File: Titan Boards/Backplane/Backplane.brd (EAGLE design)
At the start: 195.1 x 76.2 mm, 29 parts, among them P1 39-30-02?_S, P3 39-30-04?_S

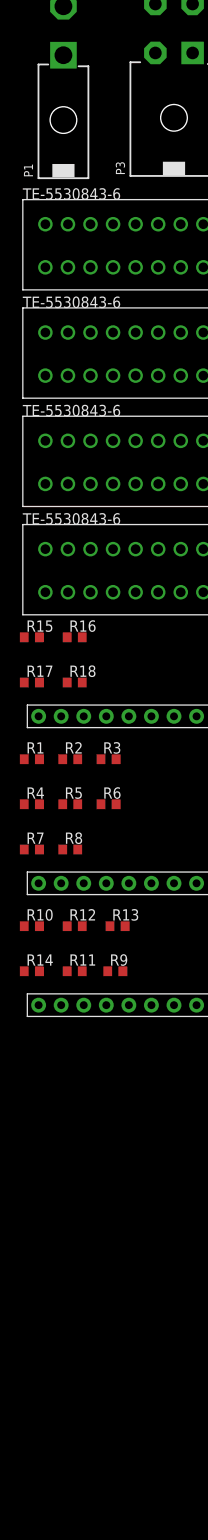
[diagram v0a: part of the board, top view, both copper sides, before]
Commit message: First final version of Titan Backplane Schematic
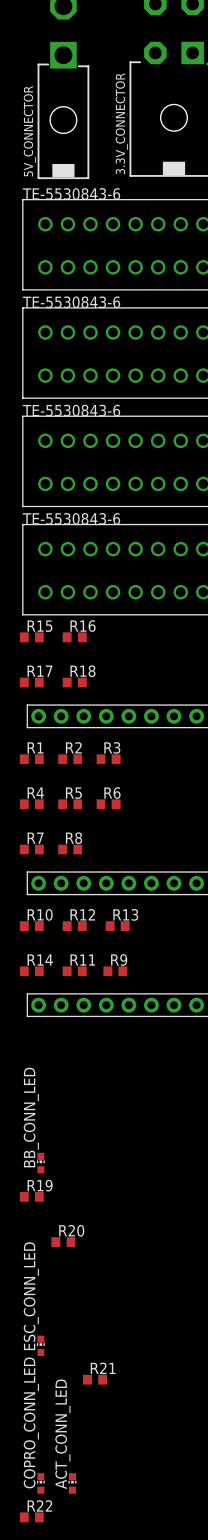
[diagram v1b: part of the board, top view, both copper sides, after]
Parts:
- added ACT_CONN_LED, BB_CONN_LED, COPRO_CONN_LED, ESC_CONN_LED: (no value), led:CHIP-LED0603
- added R19, R20, R21, R22: 36, rcl:R0603
- renumbered P1 to 5V_CONNECTOR, P3 to 3.3V_CONNECTOR, U$5 to KILLSWITCH_CONNECTOR, U$6 to THRUSTER_CONNECTOR, U$7 to ENABLE_SIGNALS_CONNECTOR, U$8 to I2C_CONNECTOR
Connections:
- removed net SPARE7: KILLSWITCH_CONNECTOR.P$1, U$1.43, U$2.43, U$3.43, U$4.43
- new net ACT_CONN: ACT_CONN_LED.A, U$4.43
- new net BB_CONN: BB_CONN_LED.A, U$1.43
- new net COPRO_CONN: COPRO_CONN_LED.A, U$3.43
- new net ESC_CONN: ESC_CONN_LED.A, U$2.43
- new net N$12: BB_CONN_LED.C, R19.1
- new net N$13: ESC_CONN_LED.C, R20.1
- new net N$14: COPRO_CONN_LED.C, R21.1
- new net N$15: ACT_CONN_LED.C, R22.1
- net GND: now also R19.2, R20.2, R21.2, R22.2

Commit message: Titan Backplane Final Version 1
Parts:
- removed 3.3V_CONNECTOR: 39-30-04?_S, con-molex-mini-fit:39-30-?04?
- removed ENABLE_SIGNALS_CONNECTOR: 929870-01-09_3, 3M_929852_Connector:929852-01-09_1ROW
- removed I2C_CONNECTOR: 929870-01-09_4, 3M_929852_Connector:929852-01-09_1ROW
- removed KILLSWITCH_CONNECTOR: 929870-01-09_1, 3M_929852_Connector:929852-01-09_1ROW
- removed R1, R10, R11, R12, R13, R14, R2, R3, R4, R5, R6, R7, R8, R9: 10k, rcl:R0603
- removed THRUSTER_CONNECTOR: 929870-01-09_2, 3M_929852_Connector:929852-01-09_1ROW
- added AUX_I2C_CONNECTOR1, ROBOT_I2C_CONNECTOR: 39-30-04?_S, con-molex-mini-fit:39-30-?04?
- added TESTPIN_CONNECTOR: 929870-01-09_4, 3M_929852_Connector:929852-01-09_1ROW
- SWITCH_CONNECTOR: value 39-30-08?_S -> 39-30-02?_S; device con-molex-mini-fit:39-30-?08? -> con-molex-mini-fit:39-30-?02?
- moved COPRO_CONN_LED 763.8 mm to (88.5, 58.7)
- moved R21 751.4 mm to (90.4, 58.3), turned to 270 degrees
- moved R19 736.0 mm to (119.1, 58.5), turned to 270 degrees
- moved BB_CONN_LED 732.3 mm to (121.0, 58.4)
- moved R22 727.9 mm to (90.3, 18.4), turned to 270 degrees
- moved ACT_CONN_LED 723.2 mm to (88.5, 18.2)
- moved ESC_CONN_LED 712.5 mm to (121.0, 17.8)
- moved R20 700.3 mm to (119.3, 17.8), turned to 270 degrees
- moved U$3 643.8 mm to (16.5, 55.9)
- moved U$1 631.0 mm to (124.5, 55.9)
- moved R17 616.9 mm to (54.7, 4.45), turned to 270 degrees
- moved R18 616.7 mm to (57.3, 4.45), turned to 270 degrees
- moved U$4 615.3 mm to (16.5, 15.2)
- moved R15 611.4 mm to (49.7, 4.45), turned to 270 degrees
- moved R16 611.2 mm to (52.2, 4.45), turned to 270 degrees
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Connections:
- net 12V_ON/OFF: no longer ENABLE_SIGNALS_CONNECTOR.P$3
- net 3.3V: now also AUX_I2C_CONNECTOR1.1, ROBOT_I2C_CONNECTOR.1, TESTPIN_CONNECTOR.P$7; no longer 3.3V_CONNECTOR.1, I2C_CONNECTOR.P$7, R10.1, R11.1, R12.1, R13.1, R14.1, R9.1
- net 3.3V_ON/OFF: no longer ENABLE_SIGNALS_CONNECTOR.P$1
- net 5V: now also SWITCH_CONNECTOR.1, TESTPIN_CONNECTOR.P$9; no longer I2C_CONNECTOR.P$9, R1.1, R2.1, R3.1, R4.1, R5.1, R6.1, R7.1, R8.1
- net 5V_ON/OFF: no longer ENABLE_SIGNALS_CONNECTOR.P$2
- net ACOUSTIC_ON/OFF: no longer ENABLE_SIGNALS_CONNECTOR.P$4
- net BACKPLANE_SCL: now also TESTPIN_CONNECTOR.P$4; no longer I2C_CONNECTOR.P$4
- net BACKPLANE_SDA: now also TESTPIN_CONNECTOR.P$3; no longer I2C_CONNECTOR.P$3
- net CONTROL_SIGNAL: no longer ENABLE_SIGNALS_CONNECTOR.P$7
- net GND: now also AUX_I2C_CONNECTOR1.3, ROBOT_I2C_CONNECTOR.3, SWITCH_CONNECTOR.2, TESTPIN_CONNECTOR.P$8; no longer 3.3V_CONNECTOR.3, ENABLE_SIGNALS_CONNECTOR.P$9, I2C_CONNECTOR.P$8, SWITCH_CONNECTOR.5
- net JETSON_ON/OFF: no longer ENABLE_SIGNALS_CONNECTOR.P$5
- net KILL_SWITCH: no longer KILLSWITCH_CONNECTOR.P$7, R9.2, SWITCH_CONNECTOR.2
- net MOBO_ON/OFF: no longer ENABLE_SIGNALS_CONNECTOR.P$6
- net PLTA_ON/OFF: no longer ENABLE_SIGNALS_CONNECTOR.P$8, SWITCH_CONNECTOR.1
- net PWM_1: no longer R1.2, THRUSTER_CONNECTOR.P$9
- net PWM_2: no longer R2.2, THRUSTER_CONNECTOR.P$8
- net PWM_3: no longer R3.2, THRUSTER_CONNECTOR.P$7
- net PWM_4: no longer R4.2, THRUSTER_CONNECTOR.P$6
- net PWM_5: no longer R5.2, THRUSTER_CONNECTOR.P$5
- net PWM_6: no longer R6.2, THRUSTER_CONNECTOR.P$4
- net PWM_7: no longer R7.2, THRUSTER_CONNECTOR.P$3
- net PWM_8: no longer R8.2, THRUSTER_CONNECTOR.P$2
- net ROBOT_SCL: now also AUX_I2C_CONNECTOR1.4, ROBOT_I2C_CONNECTOR.4, TESTPIN_CONNECTOR.P$6; no longer 3.3V_CONNECTOR.4, I2C_CONNECTOR.P$6
- net ROBOT_SDA: now also AUX_I2C_CONNECTOR1.2, ROBOT_I2C_CONNECTOR.2, TESTPIN_CONNECTOR.P$5; no longer 3.3V_CONNECTOR.2, I2C_CONNECTOR.P$5
- net SPARE2: no longer THRUSTER_CONNECTOR.P$1
- net SPARE3: now also TESTPIN_CONNECTOR.P$2; no longer I2C_CONNECTOR.P$2
- net SPARE4: now also TESTPIN_CONNECTOR.P$1; no longer I2C_CONNECTOR.P$1
- net SPARE5: no longer KILLSWITCH_CONNECTOR.P$9
- net SPARE6: no longer KILLSWITCH_CONNECTOR.P$8
- net SWITCH_1: no longer KILLSWITCH_CONNECTOR.P$6, R10.2, SWITCH_CONNECTOR.3
- net SWITCH_2: no longer KILLSWITCH_CONNECTOR.P$5, R11.2, SWITCH_CONNECTOR.4
- net SWITCH_3: no longer KILLSWITCH_CONNECTOR.P$4, R12.2, SWITCH_CONNECTOR.6
- net SWITCH_4: no longer KILLSWITCH_CONNECTOR.P$3, R13.2, SWITCH_CONNECTOR.7
- net SWITCH_5: no longer KILLSWITCH_CONNECTOR.P$2, R14.2, SWITCH_CONNECTOR.8
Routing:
- net GND: track 0.00 -> 479.0 mm, vias 0 -> 8
- net 3.3V: track 0.00 -> 335.0 mm, vias 0 -> 2
- net ROBOT_SDA: track 0.00 -> 316.8 mm, vias 0 -> 5
- net 5V: track 0.00 -> 316.1 mm, vias 0 -> 3
- net ROBOT_SCL: track 0.00 -> 311.8 mm, vias 0 -> 2
- net BACKPLANE_SDA: track 0.00 -> 296.1 mm, vias 0 -> 5
- net BACKPLANE_SCL: track 0.00 -> 295.3 mm, vias 0 -> 5
- net SPARE4: track 0.00 -> 279.8 mm, vias 0 -> 4
- net SPARE3: track 0.00 -> 279.0 mm, vias 0 -> 4
- net PLTA_ON/OFF: track 0.00 -> 273.3 mm, vias 0 -> 4
- net CONTROL_SIGNAL: track 0.00 -> 272.1 mm, vias 0 -> 4
- net 3.3V_ON/OFF: track 0.00 -> 271.1 mm, vias 0 -> 4
- net SWITCH_5: track 0.00 -> 270.2 mm, vias 0 -> 4
- net 5V_ON/OFF: track 0.00 -> 270.2 mm, vias 0 -> 4
- net SWITCH_4: track 0.00 -> 269.2 mm, vias 0 -> 4
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- added copper zone on layer 1, net 3.3V
- added copper zone on layer 1, net 5V
- added copper zone on layer 1, net GND
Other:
- board size 195.1 x 76.2 mm -> 209.6 x 76.2 mm
- board text added: "3.3V"
- board text added: "5V"
- board text added: "BPlane SCL"
- board text added: "BPlane SDA"
- board text added: "Backplane"
- board text added: "GND"
- board text added: "Robot SCL"
- board text added: "Robot SDA"
- board text added: "Spare 3"
- board text added: "Spare 4"
- board text removed: "Board Name HERE!!!"
